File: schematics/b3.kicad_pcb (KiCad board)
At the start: 2 copper layers, 19.8 x 31 mm, 40 parts, among them J1 PowerPlug, J2 GroundElectrode, J3 OutputPins, J4 InputPins1, J5 InputPins2, U1 INA128, U2 INA128, U3 INA128, U4 INA128, U5 LM321

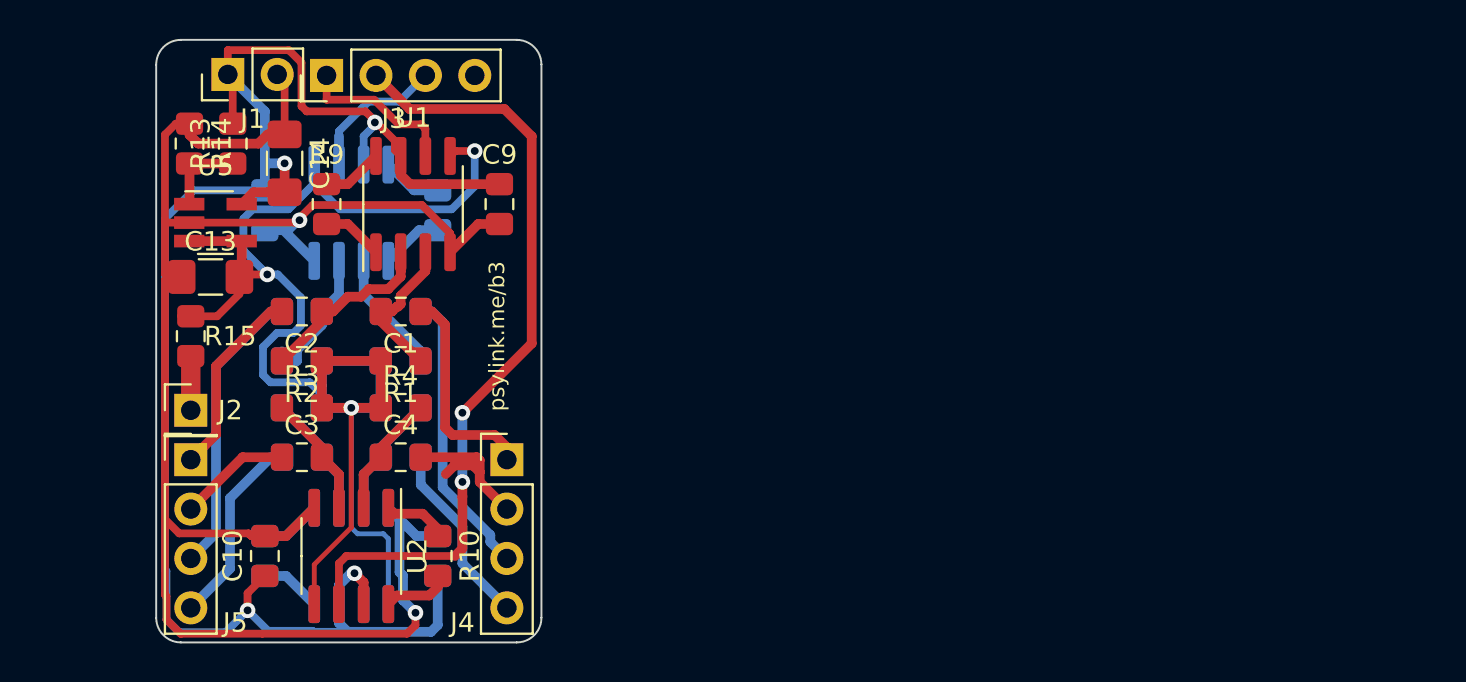
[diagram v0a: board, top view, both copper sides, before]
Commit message: finished circuit10 + board3
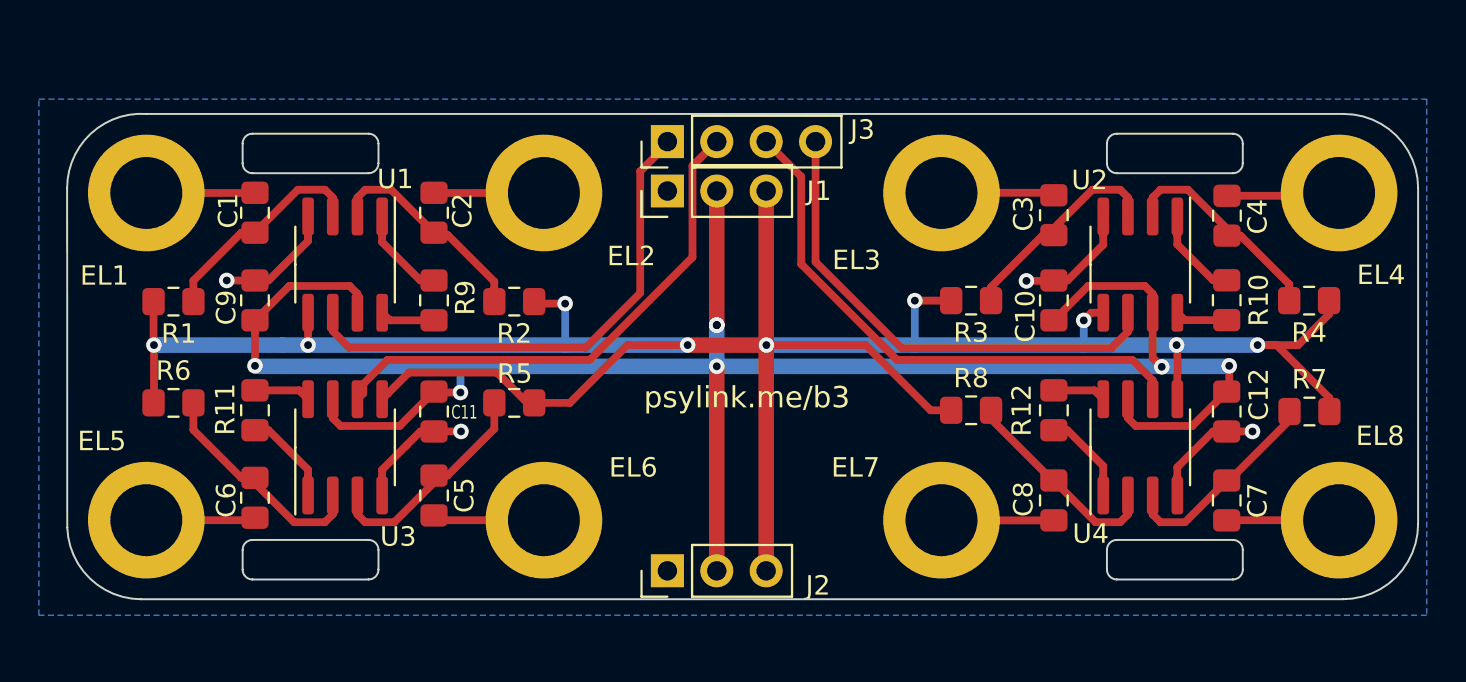
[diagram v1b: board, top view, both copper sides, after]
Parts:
- removed C13, C14: 100uF, Capacitor_SMD:C_1206_3216Metric_Pad1.42x1.75mm_HandSolder
- removed J4: InputPins1, Connector_PinHeader_2.54mm:PinHeader_1x04_P2.54mm_Vertical
- removed J5: InputPins2, Connector_PinHeader_2.54mm:PinHeader_1x04_P2.54mm_Vertical
- removed R13, R14: 100K/1%, Resistor_SMD:R_0805_2012Metric_Pad1.15x1.40mm_HandSolder
- removed R15: 100k/1%, Resistor_SMD:R_0805_2012Metric_Pad1.15x1.40mm_HandSolder
- removed U5: LM321, Package_TO_SOT_SMD:SOT-23-5_HandSoldering
- added EL1: Electrode, MountingHole:MountingHole_3.7mm_Pad, F.Cu at (29.5, 29.5)
- added EL2: Electrode, MountingHole:MountingHole_3.7mm_Pad, F.Cu at (49.9, 29.5)
- added EL3: Electrode, MountingHole:MountingHole_3.7mm_Pad, F.Cu at (70.4, 29.5)
- added EL4: Electrode, MountingHole:MountingHole_3.7mm_Pad, F.Cu at (90.8, 29.5)
- added EL5: Electrode, MountingHole:MountingHole_3.7mm_Pad, F.Cu at (29.5, 46.3)
- added EL6: Electrode, MountingHole:MountingHole_3.7mm_Pad, F.Cu at (49.9, 46.3)
- added EL7: Electrode, MountingHole:MountingHole_3.7mm_Pad, F.Cu at (70.4, 46.3)
- added EL8: Electrode, MountingHole:MountingHole_3.7mm_Pad, F.Cu at (90.8, 46.3)
- C11, C12, C5, C6, C7, C8, R11, R12, R5, R6, R7, R8, U3, U4: moved to F.Cu
- J1: value PowerPlug -> PowerInput; footprint Connector_PinHeader_2.54mm:PinHeader_1x02_P2.54mm_Vertical -> Connector_PinHeader_2.54mm:PinHeader_1x03_P2.54mm_Vertical
- J2: value GroundElectrode -> PowerPassThru; footprint Connector_PinHeader_2.54mm:PinHeader_1x01_P2.54mm_Vertical -> Connector_PinHeader_2.54mm:PinHeader_1x03_P2.54mm_Vertical
- moved R4 47.0 mm to (89.3, 35.0), turned to 180 degrees
- moved R7 46.7 mm to (89.3, 40.7), turned to 0 degrees
- moved C4 44.3 mm to (85.0, 30.6), turned to 90 degrees
- moved U2 43.3 mm to (80.6, 33.1)
- moved R10 42.7 mm to (85.0, 35.0)
- moved C10 42.7 mm to (76.1, 35.0)
- moved C7 42.5 mm to (85.0, 45.3), turned to 90 degrees
- moved R12 41.3 mm to (76.1, 40.6), turned to 90 degrees
- moved C12 41.3 mm to (85.0, 40.7), turned to 270 degrees
- moved U4 41.0 mm to (80.6, 42.5), turned to 90 degrees
- moved C3 40.6 mm to (76.1, 30.6), turned to 270 degrees
- moved C8 38.7 mm to (76.1, 45.3), turned to 270 degrees
- moved R3 34.9 mm to (71.9, 35.0), turned to 180 degrees
- moved R8 34.4 mm to (71.9, 40.6), turned to 0 degrees
- moved J2 25.9 mm to (56.3, 48.9), turned to 90 degrees
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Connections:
- C3 pad 1: /in4 -> /in3
- C4 pad 2: /in3 -> /in4
- C7 pad 1: /in7 -> /in8
- C8 pad 2: /in8 -> /in7
- J1 pad 1: VCC -> Earth
- J1 pad 2: Earth -> VCC
- J2 pad 1: /GNDtrode -> Earth
- J3 pad 2: /out2 -> /out3
- J3 pad 3: /out3 -> /out4
- J3 pad 4: /out4 -> /out2
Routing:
- net Earth: track 92.8 -> 24.7 mm, vias 2 -> 4
- net GNDS: track 87.7 -> 135.3 mm, vias 3 -> 9
- net /out4: track 0.06 -> 28.6 mm
- net /out3: track 7.35 -> 27.0 mm
- net /out1: track 8.35 -> 26.8 mm
- net VCC: track 89.7 -> 107.1 mm, vias 4 -> 7
- net /out2: track 40.7 -> 25.4 mm, vias 2 -> 0
- net /in6: track 15.0 -> 5.75 mm
- net /in5: track 14.9 -> 5.82 mm
- net Net-(C6-Pad1): track 6.35 -> 11.8 mm
- net /in1: track 11.1 -> 5.64 mm
- net Net-(C4-Pad1): track 6.36 -> 11.3 mm
- net Net-(C3-Pad2): track 6.36 -> 11.2 mm
- net Net-(C8-Pad1): track 6.35 -> 11.1 mm
- net Net-(C7-Pad2): track 6.59 -> 11.1 mm
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- added copper zone on B.Cu, net Earth
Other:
- board size 19.8 x 31 mm -> 69.5 x 25 mm
